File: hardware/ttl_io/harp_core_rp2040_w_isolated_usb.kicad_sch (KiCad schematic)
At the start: 49 parts, among them J1 Conn_01x03_Male, J2 AudioJack3, J3 USB_C_Receptacle_USB2.0, SW1 SW_Push, U1 TPD2EUSB30, U2 ADUM4160, U3 RP2040, U4 W25Q16JVUXIQ, X1 ECS-TXO-2016

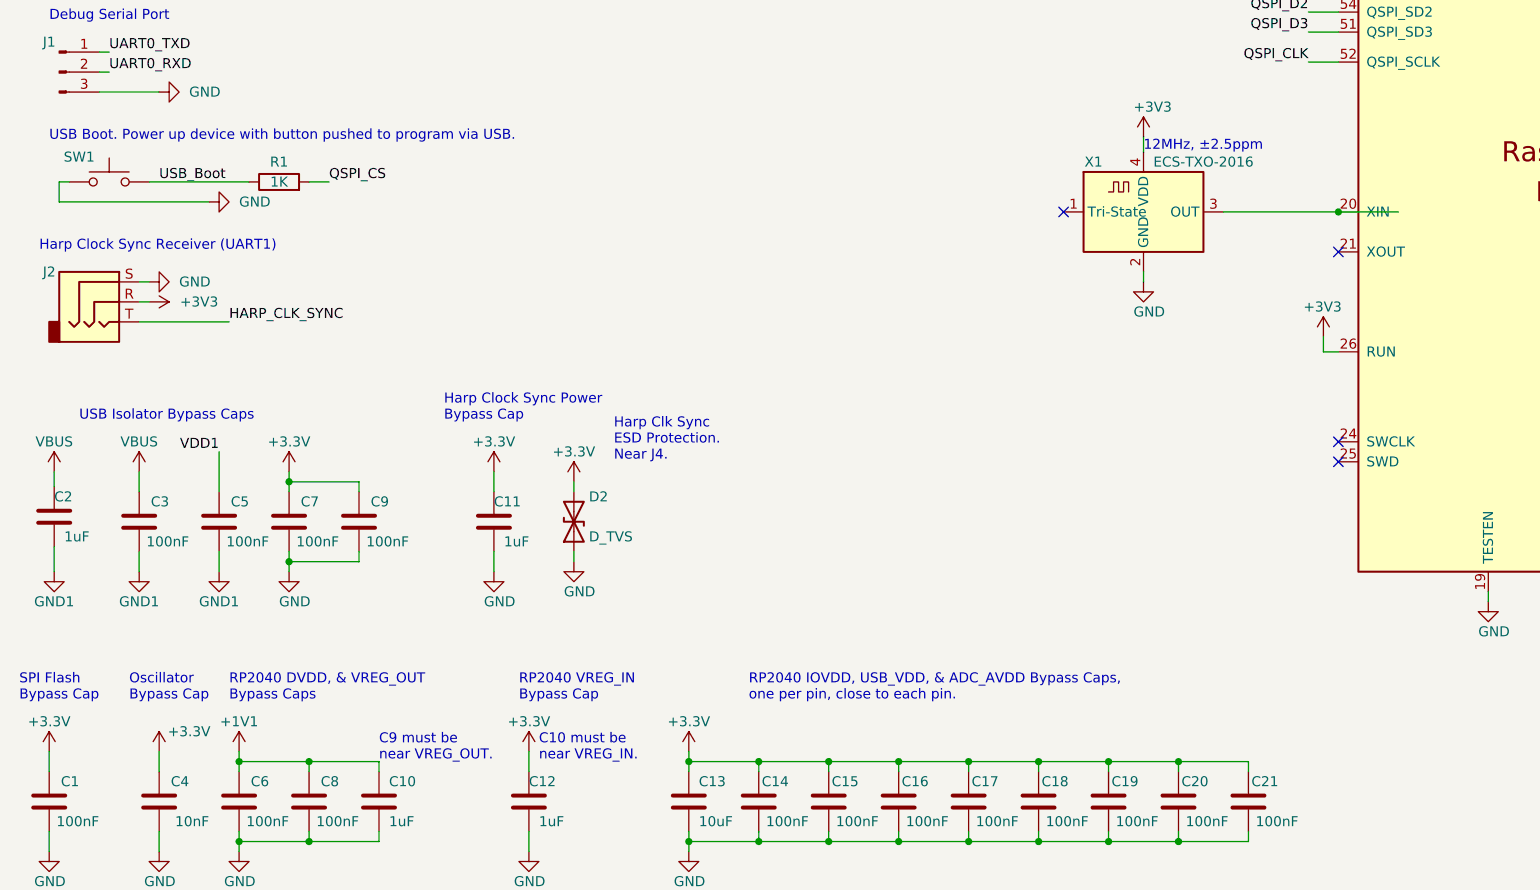
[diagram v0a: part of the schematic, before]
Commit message: draft pcb v0.1.0
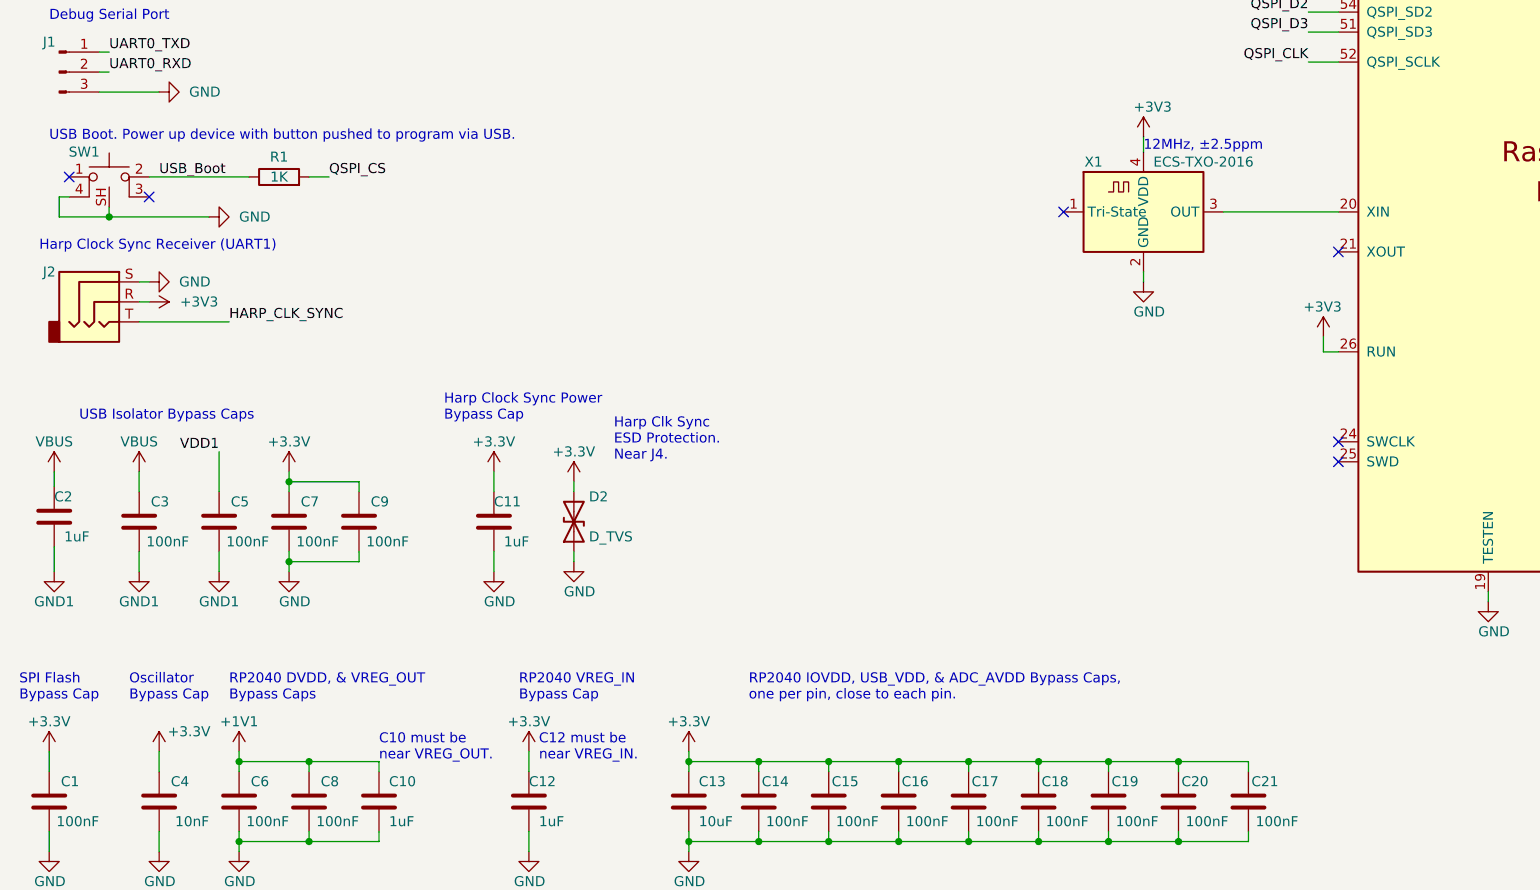
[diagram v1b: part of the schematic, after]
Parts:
- removed SW1: SW_Push, Button_Switch_SMD:SW_SPST_B3U-1000P, symbol Switch:SW_Push
- added SW1: ~, kicad_component_library:SW_Push_1P1T-SH_NO_Vertical_Wuerth_WS-TASV, symbol kicad_component_library:SW_Push_with_gnd
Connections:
- net GND: now also SW1.4, SW1.SH
- net USB_Boot: now also SW1.2
- no-connect marks 14 -> 16
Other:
- note added: "C10 must be near VREG_OUT."
- note added: "C12 must be near VREG_IN."
- note removed: "C10 must be near VREG_IN."
- note removed: "C9 must be near VREG_OUT."
- moved on the sheet: R1
